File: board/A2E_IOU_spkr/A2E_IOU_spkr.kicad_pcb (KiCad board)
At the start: 2 copper layers, 33 x 53.3 mm, 5 parts, among them J1 IOU_Socket, J2 PCB_Socket, J3 Test, U1 GAL16V8

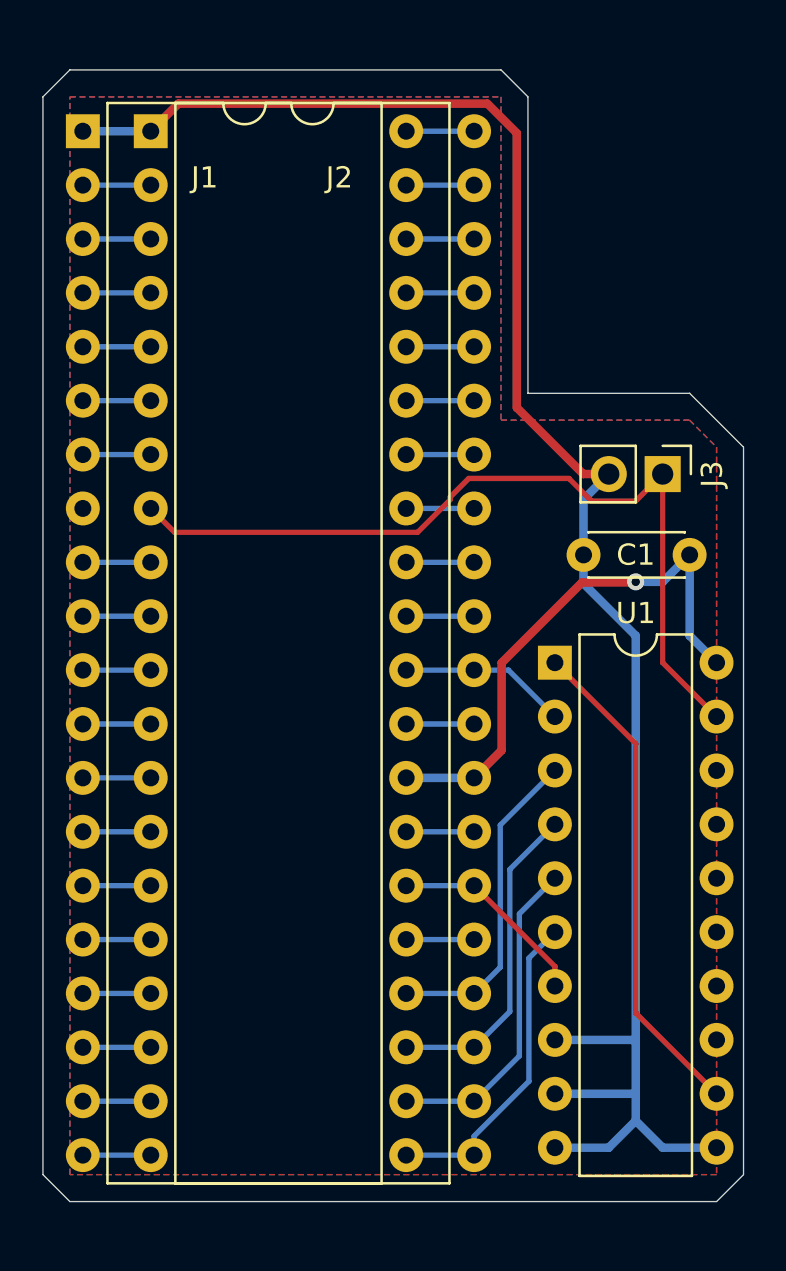
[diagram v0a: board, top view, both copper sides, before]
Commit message: Updated PCB
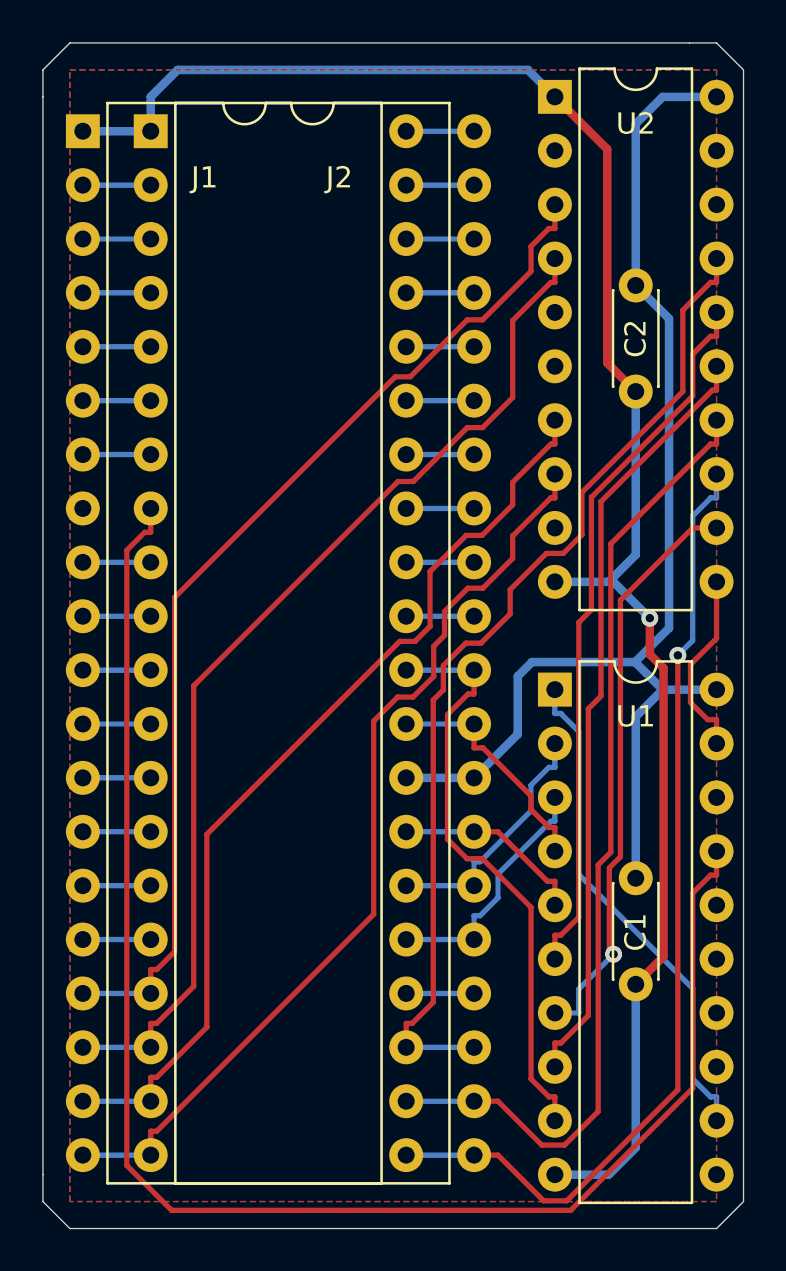
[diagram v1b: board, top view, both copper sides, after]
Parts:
- removed J3: Test, Connector_PinHeader_2.54mm:PinHeader_1x02_P2.54mm_Vertical
- added C2: 100nF, Capacitor_THT:C_Disc_D4.3mm_W1.9mm_P5.00mm, F.Cu at (64.8, 35.6)
- added U2: 74LS373, Package_DIP:DIP-20_W7.62mm, F.Cu at (61.0, 26.7)
- moved C1 15.5 mm to (64.8, 63.5), turned to 270 degrees
- moved U1 1.27 mm to (61.0, 54.6)
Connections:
- U1 pad 11: GND -> (no net)
- U1 pad 17: (no net) -> /N_SPKR
- U1 pad 19: /N_SPKR -> /ADDR_LATCH
- U1 pad 2: /~C0XX -> /PHI0
- U1 pad 3: /ORA7 -> /~PRAS
- U1 pad 4: /ORA6 -> /A6
- U1 pad 5: /ORA5 -> /Q3
- U1 pad 6: /ORA4 -> /LA7
- U1 pad 7: /PHI0 -> /LA4
- U1 pad 8: GND -> /LA5
- U1 pad 9: GND -> /~C0XX
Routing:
- net /ORA0: track 3.20 -> 49.4 mm
- net /ORA1: track 3.20 -> 49.4 mm
- net /ORA2: track 3.20 -> 44.3 mm
- net /ORA3: track 3.20 -> 44.3 mm
- net /LA5: track 0.00 -> 36.5 mm
- net /N_SPKR: track 39.2 -> 73.3 mm
- net /LA7: track 0.00 -> 34.0 mm
- net VCC: track 25.7 -> 59.5 mm, vias 1 -> 0
- net /ORA6: track 15.3 -> 47.7 mm
- net /ORA4: track 15.3 -> 45.8 mm, vias 0 -> 1
- net /ORA5: track 15.3 -> 45.6 mm
- net /LA4: track 0.00 -> 27.5 mm, vias 0 -> 1
- net /~C0XX: track 7.92 -> 27.8 mm
- net /ORA7: track 15.3 -> 3.20 mm
- net /ADDR_LATCH: track 0.00 -> 8.89 mm
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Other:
- board size 33 x 53.3 mm -> 33 x 55.9 mm
